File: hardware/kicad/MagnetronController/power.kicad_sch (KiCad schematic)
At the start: 3 parts, among them J4 Barrel_Jack_MountingPin, SW9 SW_SPST 24V

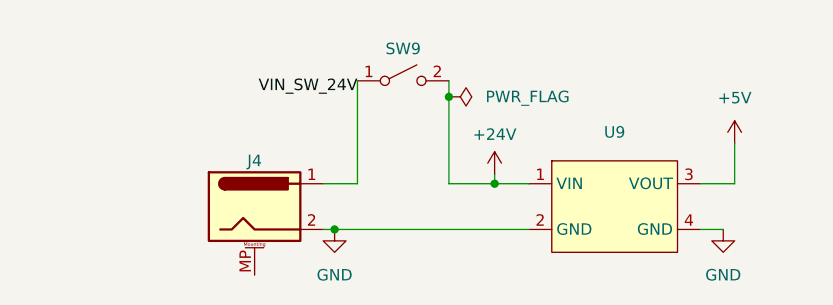
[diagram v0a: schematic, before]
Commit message: chore: cleanup
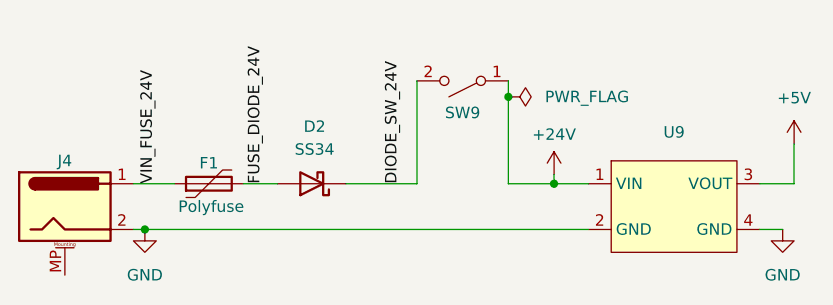
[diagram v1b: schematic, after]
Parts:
- added D2: SS34, Diode_SMD:D_SMA, symbol Diode:SS34
- added F1: Polyfuse, Fuse:Fuse_Bourns_MF-RHT300, symbol Device:Polyfuse
- SW9: footprint Connector_PinHeader_2.54mm:PinHeader_1x02_P2.54mm_Vertical -> Connector_JST:JST_XH_B2B-XH-AM_1x02_P2.50mm_Vertical
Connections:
- net +24V: now also SW9.1 (A); no longer SW9.2 (B)
- net VIN_SW_24V renamed VIN_FUSE_24V
- net VIN_FUSE_24V: now also F1.1; no longer SW9.1 (A)
- new net DIODE_SW_24V: D2.1 (K), SW9.2 (B)
- new net FUSE_DIODE_24V: D2.2 (A), F1.2
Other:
- moved on the sheet: J4, SW9, U9
